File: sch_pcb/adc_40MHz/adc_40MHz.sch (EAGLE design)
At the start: 21 parts, among them X1 BU-SMA-H, X2 BU-SMA-H

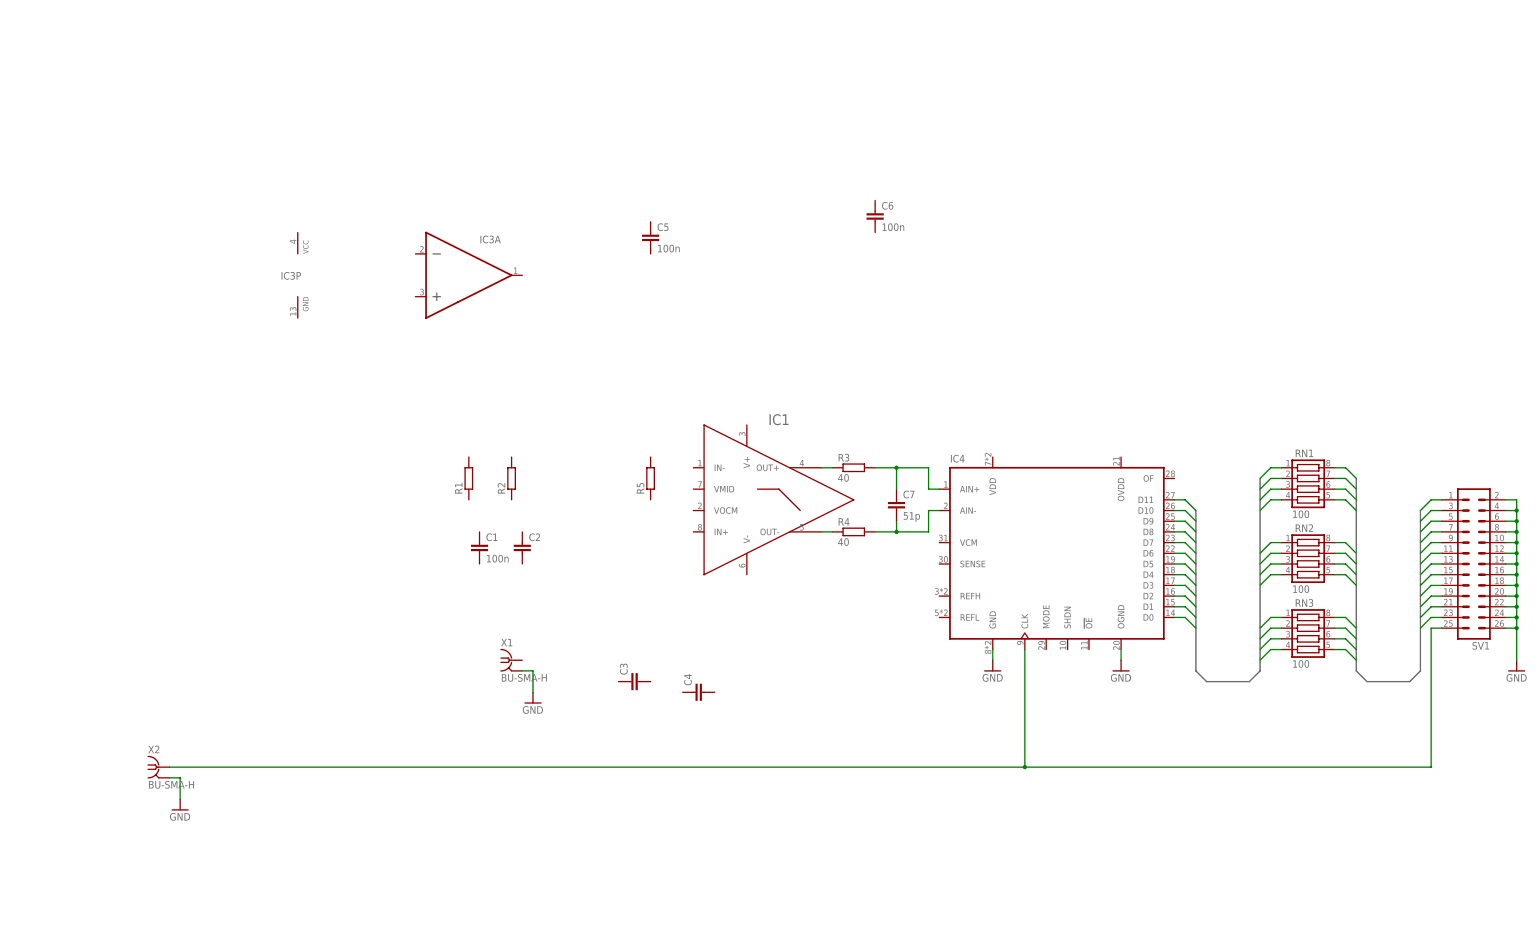
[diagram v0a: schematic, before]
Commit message: Schemat dokonczony. Do sprawdzenia. Pozostaje plytka
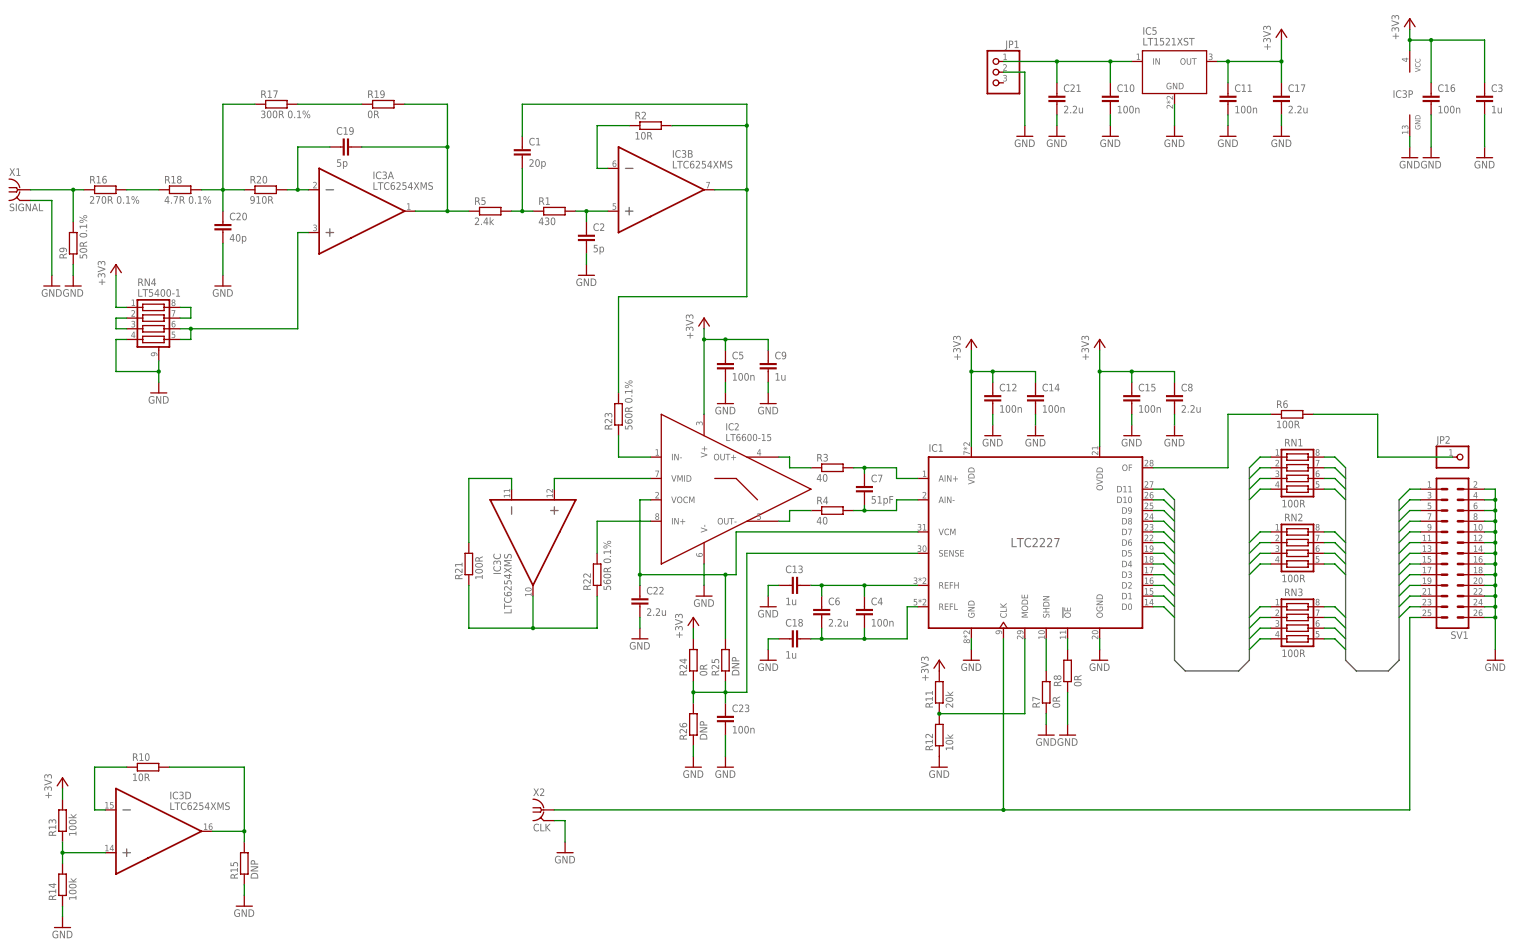
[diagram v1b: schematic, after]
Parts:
- removed IC4: (no value), ltc22xx:LTC2227
- added C10, C11, C16: 100n, rcl:C-EUC0805
- added C12, C14, C15, C23: 100n, rcl:C-EUC0603
- added C13, C18, C9: 1u, rcl:C-EUC0805
- added C17, C21, C22, C8: 2.2u, rcl:C-EUC0805
- added C19: 5p, rcl:C-EUC0603
- added C20: 40p, rcl:C-EUC0603
- added IC2: LT6600-15, lt6600:LT6600-15
- added IC5: LT1521XST, lt1521:LT1521XST
- added JP1: (no value), pinhead:PINHD-1X3/90
- added JP2: (no value), pinhead:PINHD-1X1
- added R10: 10R, rcl:R-EU_R0603
- added R11: 20k, rcl:R-EU_R0603
- added R12: 10k, rcl:R-EU_R0603
- added R13, R14: 100k, rcl:R-EU_R0603
- added R15, R25, R26: DNP, rcl:R-EU_R0603
- added R16: 270R 0.1%, rcl:R-EU_R0603
- added R17: 300R 0.1%, rcl:R-EU_R0603
- added R18: 4.7R 0.1%, rcl:R-EU_R0603
- added R19, R24, R7, R8: 0R, rcl:R-EU_R0603
- added R20: 910R, rcl:R-EU_R0603
- added R21, R6: 100R, rcl:R-EU_R0603
- added R22, R23: 560R 0.1%, rcl:R-EU_R0603
- added R9: 50R 0.1%, rcl:R-EU_R0603
- added RN4: LT5400-1, lt5400:LT5400
- C1: value 100n -> 20p
- C2: value (none) -> 5p
- C3: value (none) -> 1u
- C4: value (none) -> 100n; device rcl:C-EUC0805 -> rcl:C-EUC0603
- C6: value 100n -> 2.2u; device rcl:C-EUC0603 -> rcl:C-EUC0805
- C7: value 51p -> 51pF
- IC1: value (none) -> LTC2227; device lt6600:LT6600-15 -> ltc22xx:LTC2227
- IC3: value (none) -> LTC6254XMS
- R1: value (none) -> 430
- R2: value (none) -> 10R
- R5: value (none) -> 2.4k
- RN1, RN2, RN3: value 100 -> 100R
- X1: value BU-SMA-H -> SIGNAL
- X2: value BU-SMA-H -> CLK
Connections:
- new net +3V3: C11.1, C12.1, C14.1, C15.1, C16.1, C17.1, C3.1, C5.1, C8.1, C9.1, IC1.OVDD, IC1.VDD, IC2.V+, IC3P.V+, IC5.OUT, R11.2, R13.2, R24.2, RN4.1
- new net CLK: IC1.CLK, SV1.25, X2.1
- new net N$10: IC1.SHDN, R7.2
- new net N$11: R16.1, R9.2, X1.1
- new net N$12: IC3D.+IN, R13.1, R14.2
- new net N$13: IC3C.OUT, R21.1, R22.1
- new net N$14: IC3D.-IN, R10.1
- new net N$15: IC3D.OUT, R10.2, R15.2
- new net N$16: RN4.7, RN4.8
- new net N$17: IC3C.-IN, R21.2
- new net N$18: IC2.VMID, IC3C.+IN
- new net N$19: R16.2, R18.1
- new net N$20: C20.1, R17.1, R18.2, R20.1
- new net N$21: R17.2, R19.1
- new net N$22: C19.2, IC3A.OUT, R19.2, R5.1
- new net N$23: C19.1, IC3A.-IN, R20.2
- new net N$24: IC3A.+IN, RN4.5, RN4.6
- new net N$25: RN4.2, RN4.3
- new net N$26: IC3B.-IN, R2.1
- new net N$27: C1.1, IC3B.OUT, R2.2, R23.2
- new net N$28: C1.2, R1.1, R5.2
- new net N$29: C2.1, IC3B.+IN, R1.2
- new net N$30: IC2.IN+, R22.2
- new net N$31: IC2.IN-, R23.1
- new net N$32: IC1.MODE, R11.1, R12.2
- new net N$33: C13.2, C4.1, C6.1, IC1.REFH
- new net N$35: C23.1, IC1.SENSE, R24.1, R25.1, R26.2
- new net N$5: C22.1, IC1.VCM, IC2.VOCM, R25.2
- new net N$6: IC1.OF, R6.1
- new net N$8: JP2.1, R6.2
- new net N$9: IC1.!OE, R8.2
- new net VIN: C10.1, C21.1, IC5.IN, JP1.1
- net ADC_D0: now also IC1.D0; no longer IC4.D0
- net ADC_D1: now also IC1.D1; no longer IC4.D1
- net ADC_D10: now also IC1.D10; no longer IC4.D10
- net ADC_D11: now also IC1.D11; no longer IC4.D11
- net ADC_D2: now also IC1.D2; no longer IC4.D2
- net ADC_D3: now also IC1.D3; no longer IC4.D3
- net ADC_D4: now also IC1.D4; no longer IC4.D4
- net ADC_D5: now also IC1.D5; no longer IC4.D5
- net ADC_D6: now also IC1.D6; no longer IC4.D6
- net ADC_D7: now also IC1.D7; no longer IC4.D7
- net ADC_D8: now also IC1.D8; no longer IC4.D8
- net ADC_D9: now also IC1.D9; no longer IC4.D9
- net GND: now also C10.2, C11.2, C12.2, C13.1, C14.2, C15.2, C16.2, C17.2, C18.1, C2.2, C20.2, C21.2, C22.2, C23.2, C3.2, C5.2, C8.2, C9.2, IC1.GND, IC1.OGND, IC2.V-, IC3P.V-, IC5.GND, JP1.2, R12.1, R14.1, R15.1, R26.1, R7.1, R8.1, R9.1, RN4.4, RN4.EP; no longer IC4.OGND
- net N$1: now also IC2.OUT+; no longer IC1.OUT+
- net N$2: now also IC1.AIN+
- net N$3: now also IC1.AIN-
- net N$4: now also IC2.OUT-; no longer IC1.OUT-
- net N$7: now also C18.2, C4.2, C6.2, IC1.REFL; no longer SV1.25, X2.1
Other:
- moved on the sheet: C1, C2, C3, C4, C5, C6, C7, IC3A, IC3P, R1, R2, R3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
